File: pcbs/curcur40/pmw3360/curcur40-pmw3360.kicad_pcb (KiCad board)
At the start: 2 copper layers, 23.5 x 33 mm, 20 parts, among them J1 Conn_01x08, U1 PMW3360DM-T2QU, U2 TLV74318PDBVR

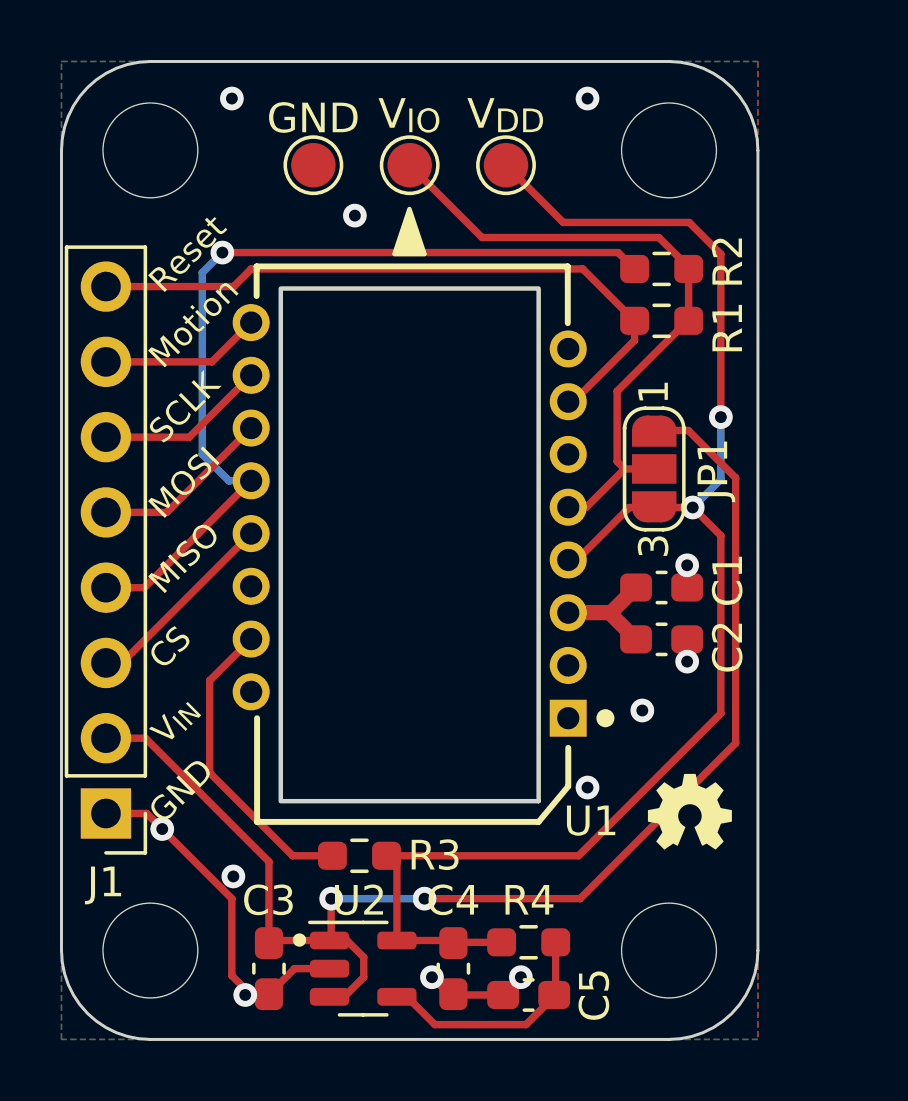
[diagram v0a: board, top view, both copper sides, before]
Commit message: fail
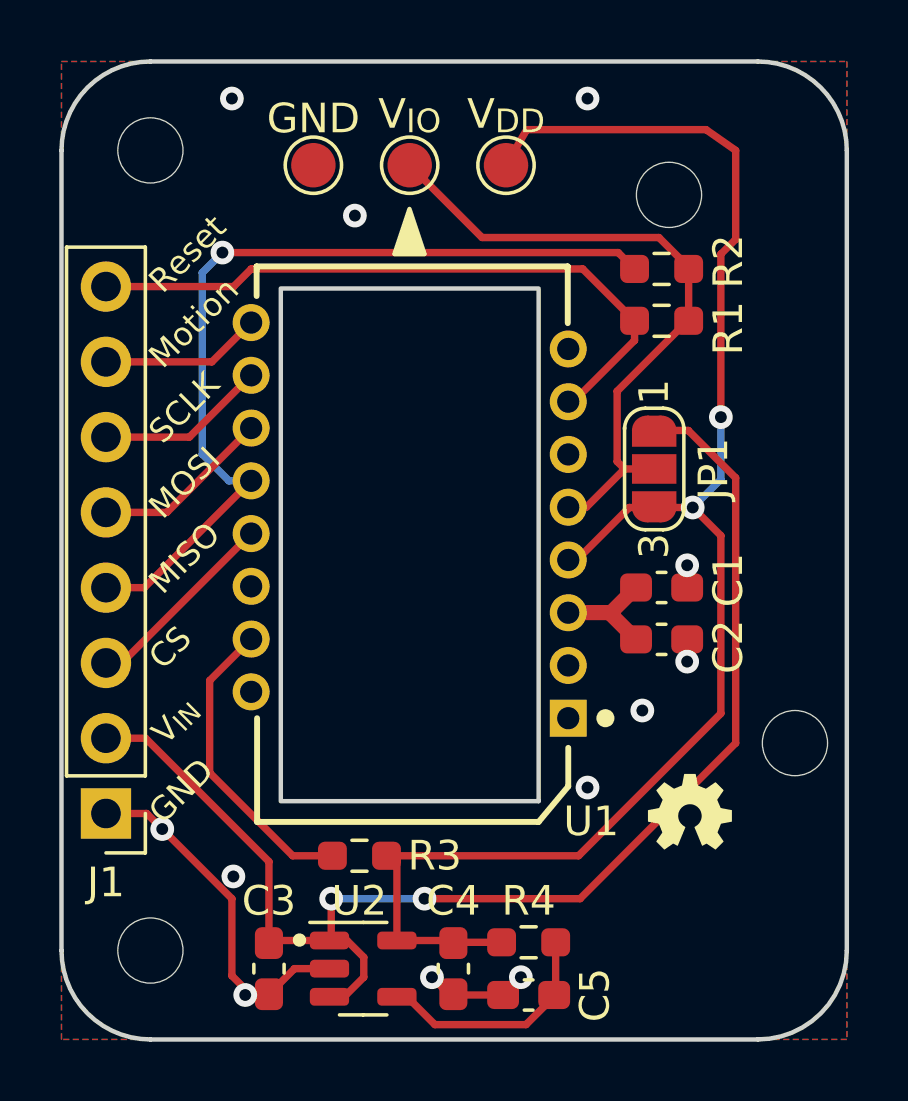
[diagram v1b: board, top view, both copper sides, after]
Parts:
- moved H4 8.19 mm to (158.6, 99.5)
- moved H3 1.50 mm to (154.4, 81.0)
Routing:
- net VDD: track 49.4 -> 53.3 mm
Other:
- board size 23.5 x 33 mm -> 26.5 x 33 mm
